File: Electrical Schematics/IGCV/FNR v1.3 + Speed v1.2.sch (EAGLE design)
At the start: 40 parts, among them IC5 DPOT, K1 35701331, K15 DF2-L-DC24V, K16 35701331, K2 DF2-L-DC24V, K3 35701331, K4 G6C-2117P, Q1 BUZ11, Q2 BUZ11, Q4 BUZ11, SW2 Pedal MS, SW3 Pedal MS, SW5 Pedal MS

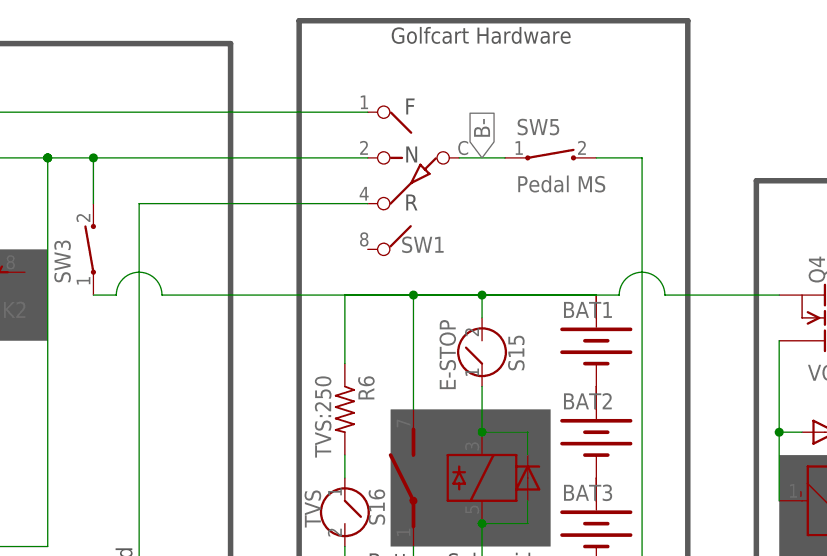
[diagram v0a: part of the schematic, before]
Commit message: Updated schematics
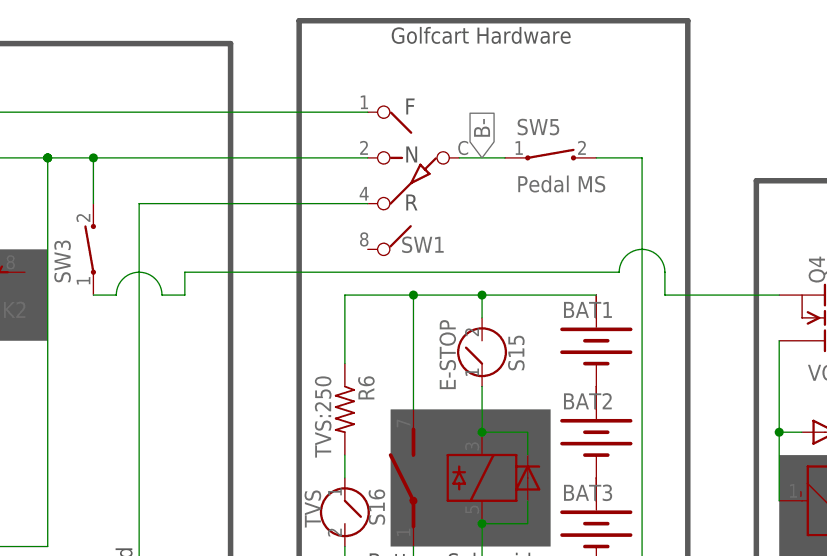
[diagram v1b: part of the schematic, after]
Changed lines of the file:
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@@
 <net name="N$4" class="0">
 <segment>
+<wire x1="134.62" y1="93.98" x2="129.54" y2="93.98" width="0.1524" layer="91" curve="180"/>
+<wire x1="134.62" y1="93.98" x2="134.62" y2="91.44" width="0.1524" layer="91"/>
 <pinref part="Q4" gate="G$1" pin="S"/>
 <wire x1="134.62" y1="91.44" x2="147.32" y2="91.44" width="0.1524" layer="91"/>
-<wire x1="134.62" y1="91.44" x2="129.54" y2="91.44" width="0.1524" layer="91" curve="180"/>
-<wire x1="129.54" y1="91.44" x2="78.74" y2="91.44" width="0.1524" layer="91"/>
+<wire x1="129.54" y1="93.98" x2="81.28" y2="93.98" width="0.1524" layer="91"/>
+<wire x1="81.28" y1="93.98" x2="81.28" y2="91.44" width="0.1524" layer="91"/>
+<wire x1="73.66" y1="91.44" x2="78.74" y2="91.44" width="0.1524" layer="91" curve="-180"/>
 <pinref part="SW3" gate="G$1" pin="1"/>
 <wire x1="71.12" y1="91.44" x2="73.66" y2="91.44" width="0.1524" layer="91"/>
-<wire x1="73.66" y1="91.44" x2="78.74" y2="91.44" width="0.1524" layer="91" curve="-180"/>
+<wire x1="81.28" y1="91.44" x2="78.74" y2="91.44" width="0.1524" layer="91"/>
 </segment>
 </net>
